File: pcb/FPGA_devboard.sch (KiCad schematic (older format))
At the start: 2 parts, among them X3 AC7020, X4 Conn_02x05_Odd_Even

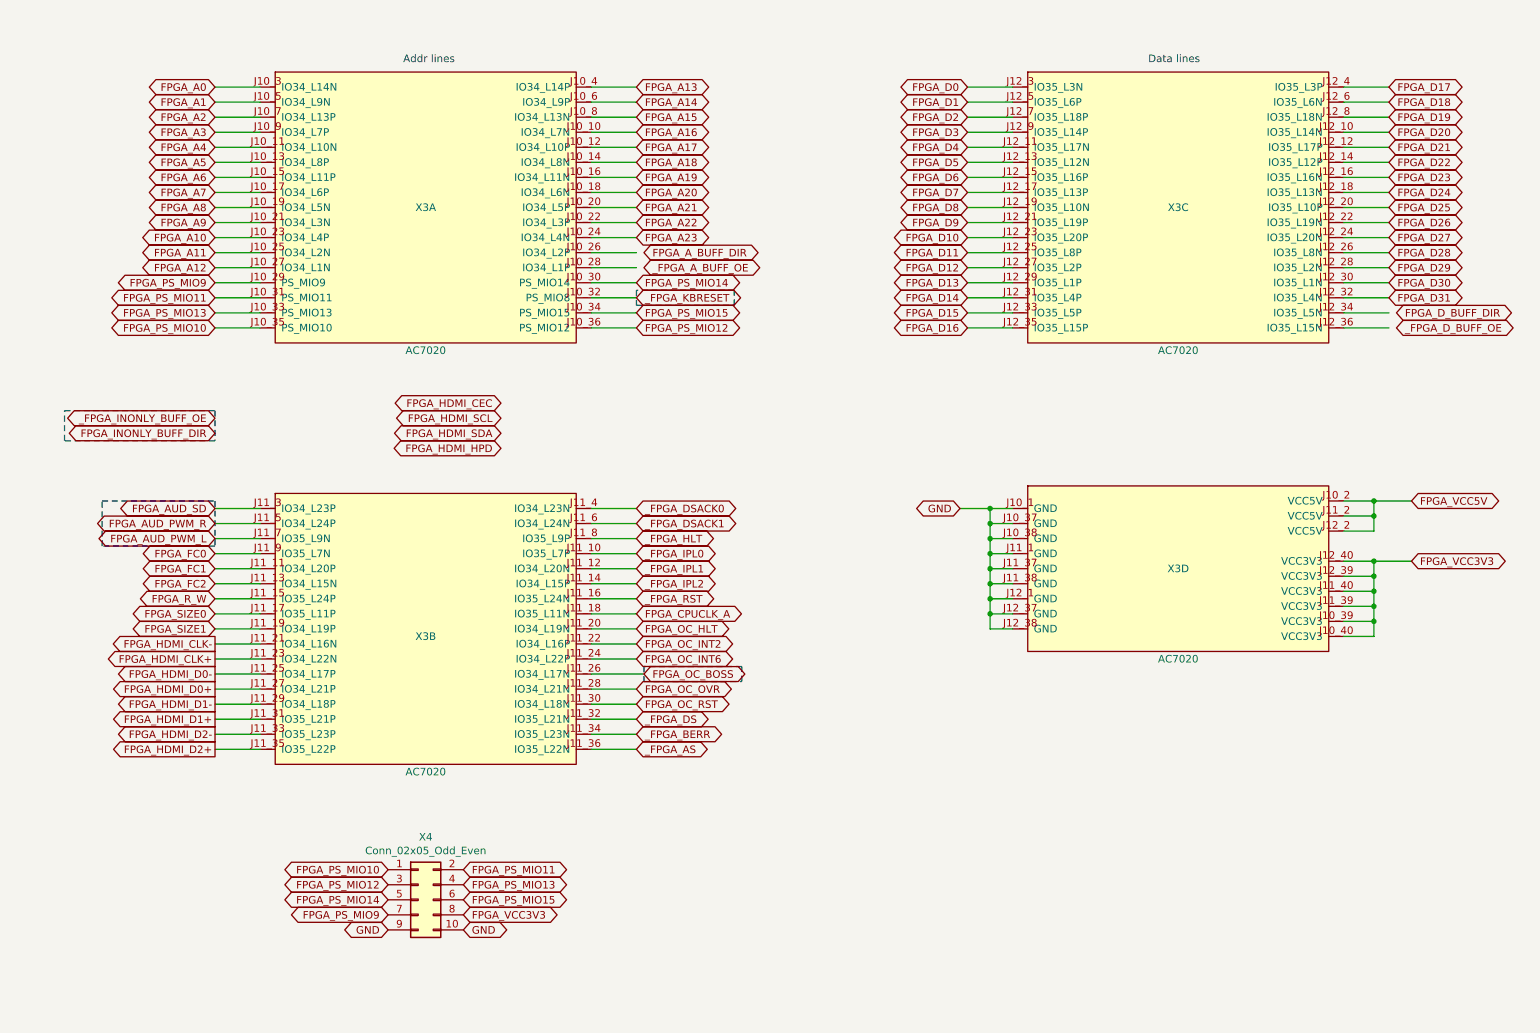
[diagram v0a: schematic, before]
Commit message: some dirty routing
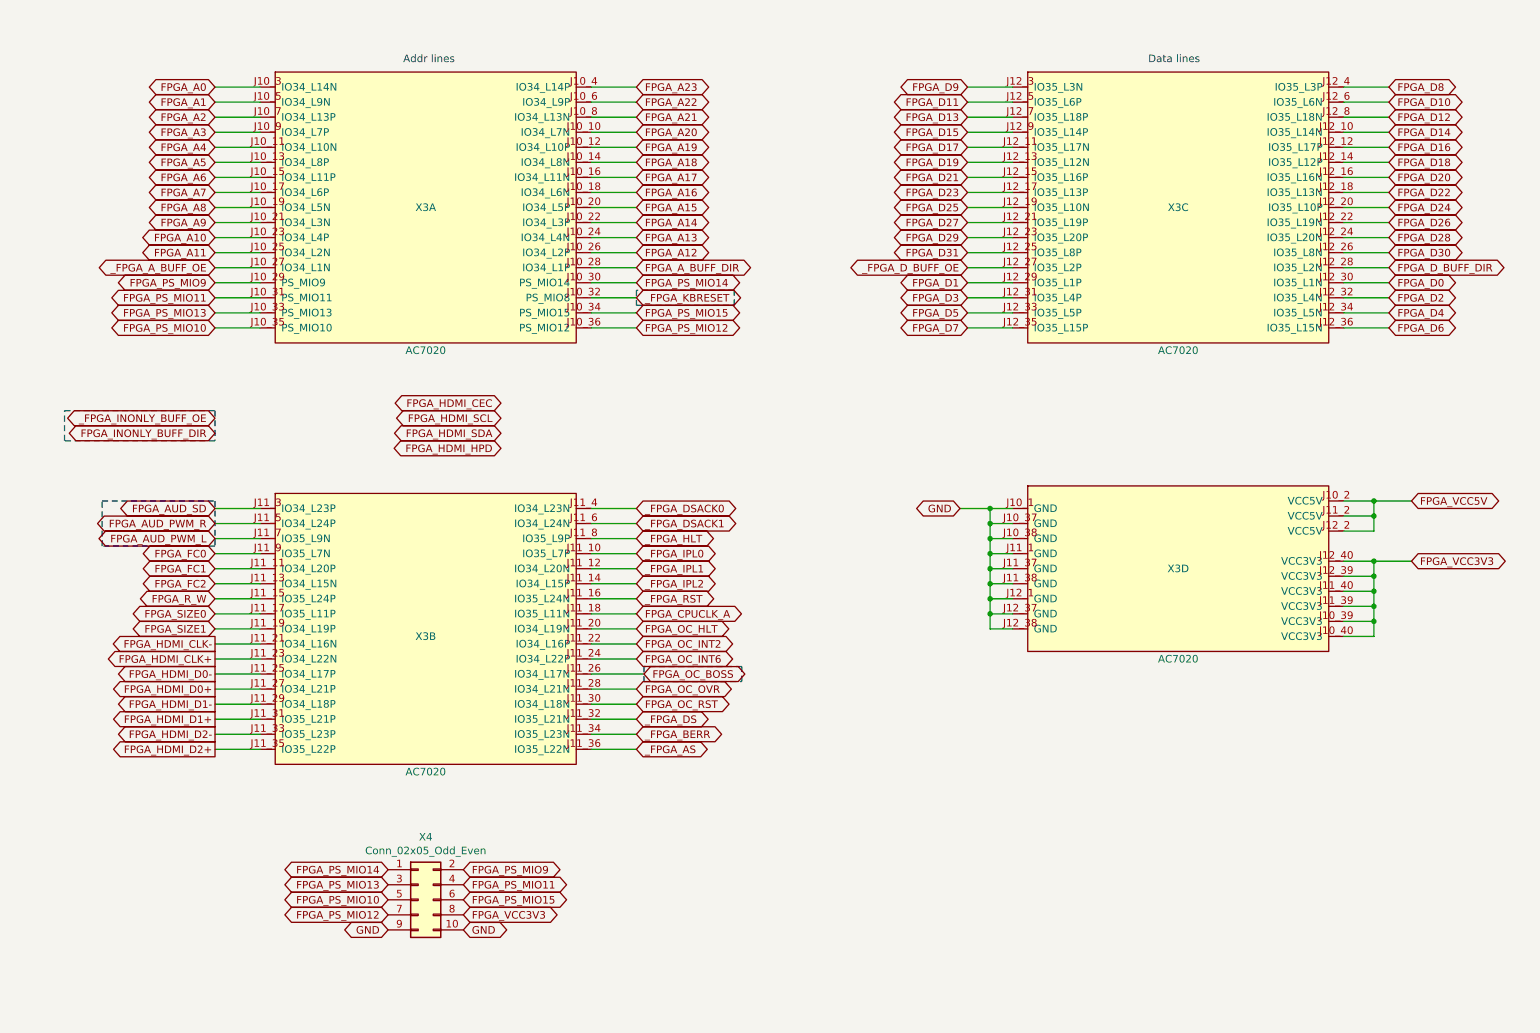
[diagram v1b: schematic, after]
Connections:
- net FPGA_A12: now also X3.J10_26 (IO34_L2P); no longer X3.J10_27 (IO34_L1N)
- net FPGA_A13: now also X3.J10_24 (IO34_L4N); no longer X3.J10_4 (IO34_L14P)
- net FPGA_A14: now also X3.J10_22 (IO34_L3P); no longer X3.J10_6 (IO34_L9P)
- net FPGA_A15: now also X3.J10_20 (IO34_L5P); no longer X3.J10_8 (IO34_L13N)
- net FPGA_A16: now also X3.J10_18 (IO34_L6N); no longer X3.J10_10 (IO34_L7N)
- net FPGA_A17: now also X3.J10_16 (IO34_L11N); no longer X3.J10_12 (IO34_L10P)
- net FPGA_A19: now also X3.J10_12 (IO34_L10P); no longer X3.J10_16 (IO34_L11N)
- net FPGA_A20: now also X3.J10_10 (IO34_L7N); no longer X3.J10_18 (IO34_L6N)
- net FPGA_A21: now also X3.J10_8 (IO34_L13N); no longer X3.J10_20 (IO34_L5P)
- net FPGA_A22: now also X3.J10_6 (IO34_L9P); no longer X3.J10_22 (IO34_L3P)
- net FPGA_A23: now also X3.J10_4 (IO34_L14P); no longer X3.J10_24 (IO34_L4N)
- net FPGA_A_BUFF_DIR: now also X3.J10_28 (IO34_L1P)
- net FPGA_D0: now also X3.J12_30 (IO35_L1N); no longer X3.J12_3 (IO35_L3N)
- net FPGA_D1: now also X3.J12_29 (IO35_L1P); no longer X3.J12_5 (IO35_L6P)
- net FPGA_D10: now also X3.J12_6 (IO35_L6N); no longer X3.J12_23 (IO35_L20P)
- net FPGA_D11: now also X3.J12_5 (IO35_L6P); no longer X3.J12_25 (IO35_L8P)
- net FPGA_D12: now also X3.J12_8 (IO35_L18N); no longer X3.J12_27 (IO35_L2P)
- net FPGA_D13: now also X3.J12_7 (IO35_L18P); no longer X3.J12_29 (IO35_L1P)
- net FPGA_D14: now also X3.J12_10 (IO35_L14N); no longer X3.J12_31 (IO35_L4P)
- net FPGA_D15: now also X3.J12_9 (IO35_L14P); no longer X3.J12_33 (IO35_L5P)
- net FPGA_D16: now also X3.J12_12 (IO35_L17P); no longer X3.J12_35 (IO35_L15P)
- net FPGA_D17: now also X3.J12_11 (IO35_L17N); no longer X3.J12_4 (IO35_L3P)
- net FPGA_D18: now also X3.J12_14 (IO35_L12P); no longer X3.J12_6 (IO35_L6N)
- net FPGA_D19: now also X3.J12_13 (IO35_L12N); no longer X3.J12_8 (IO35_L18N)
- net FPGA_D2: now also X3.J12_32 (IO35_L4N); no longer X3.J12_7 (IO35_L18P)
- net FPGA_D20: now also X3.J12_16 (IO35_L16N); no longer X3.J12_10 (IO35_L14N)
- net FPGA_D21: now also X3.J12_15 (IO35_L16P); no longer X3.J12_12 (IO35_L17P)
- net FPGA_D22: now also X3.J12_18 (IO35_L13N); no longer X3.J12_14 (IO35_L12P)
- net FPGA_D23: now also X3.J12_17 (IO35_L13P); no longer X3.J12_16 (IO35_L16N)
- net FPGA_D24: now also X3.J12_20 (IO35_L10P); no longer X3.J12_18 (IO35_L13N)
- net FPGA_D25: now also X3.J12_19 (IO35_L10N); no longer X3.J12_20 (IO35_L10P)
- net FPGA_D27: now also X3.J12_21 (IO35_L19P); no longer X3.J12_24 (IO35_L20N)
- net FPGA_D28: now also X3.J12_24 (IO35_L20N); no longer X3.J12_26 (IO35_L8N)
- net FPGA_D29: now also X3.J12_23 (IO35_L20P); no longer X3.J12_28 (IO35_L2N)
- net FPGA_D3: now also X3.J12_31 (IO35_L4P); no longer X3.J12_9 (IO35_L14P)
- net FPGA_D30: now also X3.J12_26 (IO35_L8N); no longer X3.J12_30 (IO35_L1N)
- net FPGA_D31: now also X3.J12_25 (IO35_L8P); no longer X3.J12_32 (IO35_L4N)
- net FPGA_D4: now also X3.J12_34 (IO35_L5N); no longer X3.J12_11 (IO35_L17N)
- net FPGA_D5: now also X3.J12_33 (IO35_L5P); no longer X3.J12_13 (IO35_L12N)
- net FPGA_D6: now also X3.J12_36 (IO35_L15N); no longer X3.J12_15 (IO35_L16P)
- net FPGA_D7: now also X3.J12_35 (IO35_L15P); no longer X3.J12_17 (IO35_L13P)
- net FPGA_D8: now also X3.J12_4 (IO35_L3P); no longer X3.J12_19 (IO35_L10N)
- net FPGA_D9: now also X3.J12_3 (IO35_L3N); no longer X3.J12_21 (IO35_L19P)
- net FPGA_D_BUFF_DIR: now also X3.J12_28 (IO35_L2N)
- net FPGA_PS_MIO10: now also X4.5 (Pin_5); no longer X4.1 (Pin_1)
- net FPGA_PS_MIO11: now also X4.4 (Pin_4); no longer X4.2 (Pin_2)
- net FPGA_PS_MIO12: now also X4.7 (Pin_7); no longer X4.3 (Pin_3)
- net FPGA_PS_MIO13: now also X4.3 (Pin_3); no longer X4.4 (Pin_4)
- net FPGA_PS_MIO14: now also X4.1 (Pin_1); no longer X4.5 (Pin_5)
- net FPGA_PS_MIO9: now also X4.2 (Pin_2); no longer X4.7 (Pin_7)
- net _FPGA_A_BUFF_OE: now also X3.J10_27 (IO34_L1N)
- net _FPGA_D_BUFF_OE: now also X3.J12_27 (IO35_L2P)
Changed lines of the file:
@@
 Text GLabel 1800 2700 0    50   BiDi ~ 0
 FPGA_A11
-Text GLabel 1800 2800 0    50   BiDi ~ 0
+Text GLabel 4600 2700 2    50   BiDi ~ 0
 FPGA_A12
-Text GLabel 4600 1600 2    50   BiDi ~ 0
+Text GLabel 4600 2600 2    50   BiDi ~ 0
 FPGA_A13
-Text GLabel 4600 1700 2    50   BiDi ~ 0
+Text GLabel 4600 2500 2    50   BiDi ~ 0
 FPGA_A14
-Text GLabel 4600 1800 2    50   BiDi ~ 0
+Text GLabel 4600 2400 2    50   BiDi ~ 0
 FPGA_A15
-Text GLabel 4600 1900 2    50   BiDi ~ 0
+Text GLabel 4600 2300 2    50   BiDi ~ 0
 FPGA_A16
-Text GLabel 4600 2000 2    50   BiDi ~ 0
+Text GLabel 4600 2200 2    50   BiDi ~ 0
 FPGA_A17
 Text GLabel 4600 2100 2    50   BiDi ~ 0
 FPGA_A18
-Text GLabel 4600 2200 2    50   BiDi ~ 0
+Text GLabel 4600 2000 2    50   BiDi ~ 0
 FPGA_A19
-Text GLabel 4600 2300 2    50   BiDi ~ 0
+Text GLabel 4600 1900 2    50   BiDi ~ 0
 FPGA_A20
-Text GLabel 4600 2400 2    50   BiDi ~ 0
+Text GLabel 4600 1800 2    50   BiDi ~ 0
 FPGA_A21
-Text GLabel 4600 2500 2    50   BiDi ~ 0
+Text GLabel 4600 1700 2    50   BiDi ~ 0
 FPGA_A22
-Text GLabel 4600 2600 2    50   BiDi ~ 0
+Text GLabel 4600 1600 2    50   BiDi ~ 0
 FPGA_A23
-Text GLabel 4650 2700 2    50   BiDi ~ 0
+Text GLabel 4600 2800 2    50   BiDi ~ 0
 FPGA_A_BUFF_DIR
-Text GLabel 4650 2800 2    50   BiDi ~ 0
+Text GLabel 1800 2800 0    50   BiDi ~ 0
 _FPGA_A_BUFF_OE
+Text GLabel 9600 2900 2    50   BiDi ~ 0
+FPGA_D0
+Text GLabel 6800 2900 0    50   BiDi ~ 0
+FPGA_D1
+Text GLabel 9600 3000 2    50   BiDi ~ 0
+FPGA_D2
+Text GLabel 6800 3000 0    50   BiDi ~ 0
+FPGA_D3
+Text GLabel 9600 3100 2    50   BiDi ~ 0
+FPGA_D4
+Text GLabel 6800 3100 0    50   BiDi ~ 0
+FPGA_D5
+Text GLabel 9600 3200 2    50   BiDi ~ 0
+FPGA_D6
+Text GLabel 6800 3200 0    50   BiDi ~ 0
+FPGA_D7
+Text GLabel 9600 1600 2    50   BiDi ~ 0
+FPGA_D8
 Text GLabel 6800 1600 0    50   BiDi ~ 0
-FPGA_D0
+FPGA_D9
+Text GLabel 9600 1700 2    50   BiDi ~ 0
+FPGA_D10
 Text GLabel 6800 1700 0    50   BiDi ~ 0
-FPGA_D1
+FPGA_D11
+Text GLabel 9600 1800 2    50   BiDi ~ 0
+FPGA_D12
 Text GLabel 6800 1800 0    50   BiDi ~ 0
-FPGA_D2
+FPGA_D13
+Text GLabel 9600 1900 2    50   BiDi ~ 0
+FPGA_D14
 Text GLabel 6800 1900 0    50   BiDi ~ 0
-FPGA_D3
+FPGA_D15
+Text GLabel 9600 2000 2    50   BiDi ~ 0
+FPGA_D16
 Text GLabel 6800 2000 0    50   BiDi ~ 0
-FPGA_D4
+FPGA_D17
+Text GLabel 9600 2100 2    50   BiDi ~ 0
+FPGA_D18
 Text GLabel 6800 2100 0    50   BiDi ~ 0
-FPGA_D5
+FPGA_D19
+Text GLabel 9600 2200 2    50   BiDi ~ 0
+FPGA_D20
 Text GLabel 6800 2200 0    50   BiDi ~ 0
-FPGA_D6
+FPGA_D21
+Text GLabel 9600 2300 2    50   BiDi ~ 0
+FPGA_D22
 Text GLabel 6800 2300 0    50   BiDi ~ 0
-FPGA_D7
+FPGA_D23
+Text GLabel 9600 2400 2    50   BiDi ~ 0
+FPGA_D24
 Text GLabel 6800 2400 0    50   BiDi ~ 0
-FPGA_D8
-Text GLabel 6800 2500 0    50   BiDi ~ 0
-FPGA_D9
-Text GLabel 6800 2600 0    50   BiDi ~ 0
-FPGA_D10
-Text GLabel 6800 2700 0    50   BiDi ~ 0
-FPGA_D11
-Text GLabel 6800 2800 0    50   BiDi ~ 0
-FPGA_D12
-Text GLabel 6800 2900 0    50   BiDi ~ 0
-FPGA_D13
-Text GLabel 6800 3000 0    50   BiDi ~ 0
-FPGA_D14
-Text GLabel 6800 3100 0    50   BiDi ~ 0
-FPGA_D15
-Text GLabel 6800 3200 0    50   BiDi ~ 0
-FPGA_D16
-Text GLabel 9600 1600 2    50   BiDi ~ 0
-FPGA_D17
-Text GLabel 9600 1700 2    50   BiDi ~ 0
-FPGA_D18
-Text GLabel 9600 1800 2    50   BiDi ~ 0
-FPGA_D19
-Text GLabel 9600 1900 2    50   BiDi ~ 0
-FPGA_D20
-Text GLabel 9600 2000 2    50   BiDi ~ 0
-FPGA_D21
-Text GLabel 9600 2100 2    50   BiDi ~ 0
-FPGA_D22
-Text GLabel 9600 2200 2    50   BiDi ~ 0
-FPGA_D23
-Text GLabel 9600 2300 2    50   BiDi ~ 0
-FPGA_D24
-Text GLabel 9600 2400 2    50   BiDi ~ 0
 FPGA_D25
 Text GLabel 9600 2500 2    50   BiDi ~ 0
 FPGA_D26
+Text GLabel 6800 2500 0    50   BiDi ~ 0
+FPGA_D27
 Text GLabel 9600 2600 2    50   BiDi ~ 0
-FPGA_D27
+FPGA_D28
+Text GLabel 6800 2600 0    50   BiDi ~ 0
+FPGA_D29
 Text GLabel 9600 2700 2    50   BiDi ~ 0
-FPGA_D28
+FPGA_D30
+Text GLabel 6800 2700 0    50   BiDi ~ 0
+FPGA_D31
 Text GLabel 9600 2800 2    50   BiDi ~ 0
-FPGA_D29
-Text GLabel 9600 2900 2    50   BiDi ~ 0
-FPGA_D30
-Text GLabel 9600 3000 2    50   BiDi ~ 0
-FPGA_D31
-Text GLabel 9650 3100 2    50   BiDi ~ 0
 FPGA_D_BUFF_DIR
-Text GLabel 9650 3200 2    50   BiDi ~ 0
+Text GLabel 6800 2800 0    50   BiDi ~ 0
 _FPGA_D_BUFF_OE
 Text GLabel 1800 4600 0    50   BiDi ~ 0
@@
 Text GLabel 3450 7100 2    50   BiDi ~ 0
 FPGA_VCC3V3
-Text GLabel 1800 3000 0    50   BiDi ~ 0
-FPGA_PS_MIO11
 Text GLabel 1800 3100 0    50   BiDi ~ 0
 FPGA_PS_MIO13
@@
 Text GLabel 4600 2900 2    50   BiDi ~ 0
 FPGA_PS_MIO14
+Text GLabel 2950 7000 0    50   BiDi ~ 0
+FPGA_PS_MIO10
+Text GLabel 3450 6900 2    50   BiDi ~ 0
+FPGA_PS_MIO11
+Text GLabel 2950 7100 0    50   BiDi ~ 0
+FPGA_PS_MIO12
+Text GLabel 2950 6900 0    50   BiDi ~ 0
+FPGA_PS_MIO13
 Text GLabel 2950 6800 0    50   BiDi ~ 0
-FPGA_PS_MIO10
-Text GLabel 3450 6800 2    50   BiDi ~ 0
-FPGA_PS_MIO11
-Text GLabel 2950 6900 0    50   BiDi ~ 0
-FPGA_PS_MIO12
-Text GLabel 3450 6900 2    50   BiDi ~ 0
-FPGA_PS_MIO13
-Text GLabel 2950 7000 0    50   BiDi ~ 0
 FPGA_PS_MIO14
 Text GLabel 3450 7000 2    50   BiDi ~ 0
@@
 Wire Notes Line
 	4600 3050 5250 3050
-Wire Notes Line
-	5250 3050 5250 2950
-Wire Notes Line
-	5250 2950 4600 2950
 Text GLabel 1800 6000 0    50   Output ~ 0
 FPGA_HDMI_D2+
@@
 Wire Wire Line
 	1800 2900 2100 2900
-Text GLabel 4600 3000 2    50   BiDi ~ 0
-_FPGA_KBRESET
 Wire Notes Line
 	4600 2950 4600 3050
@@
 Wire Wire Line
 	4300 5500 4650 5500
-Text GLabel 2950 7100 0    50   BiDi ~ 0
+Text GLabel 3450 6800 2    50   BiDi ~ 0
 FPGA_PS_MIO9
 Text GLabel 1800 2900 0    50   BiDi ~ 0
@@
 Wire Wire Line
 	4300 3000 4600 3000
+Text GLabel 1800 3000 0    50   BiDi ~ 0
+FPGA_PS_MIO11
+Text GLabel 4600 3000 2    50   BiDi ~ 0
+_FPGA_KBRESET
+Wire Notes Line
+	5250 2950 4600 2950
+Wire Notes Line
+	5250 3050 5250 2950
 $EndSCHEMATC
